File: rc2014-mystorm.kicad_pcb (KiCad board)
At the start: 2 copper layers, 100 x 50 mm, 25 parts, among them J1 FPGA connection, J2 Config, J3 Conn_01x05, J6 Extra, P1 RC2014 BUS, U1 SN74LVCC3245A, U2 SN74LVCC3245A, U3 SN74LVCC3245A, U4 SN74LVCC3245A, U5 SN74LVCC3245A, U6 LM1117-3.3

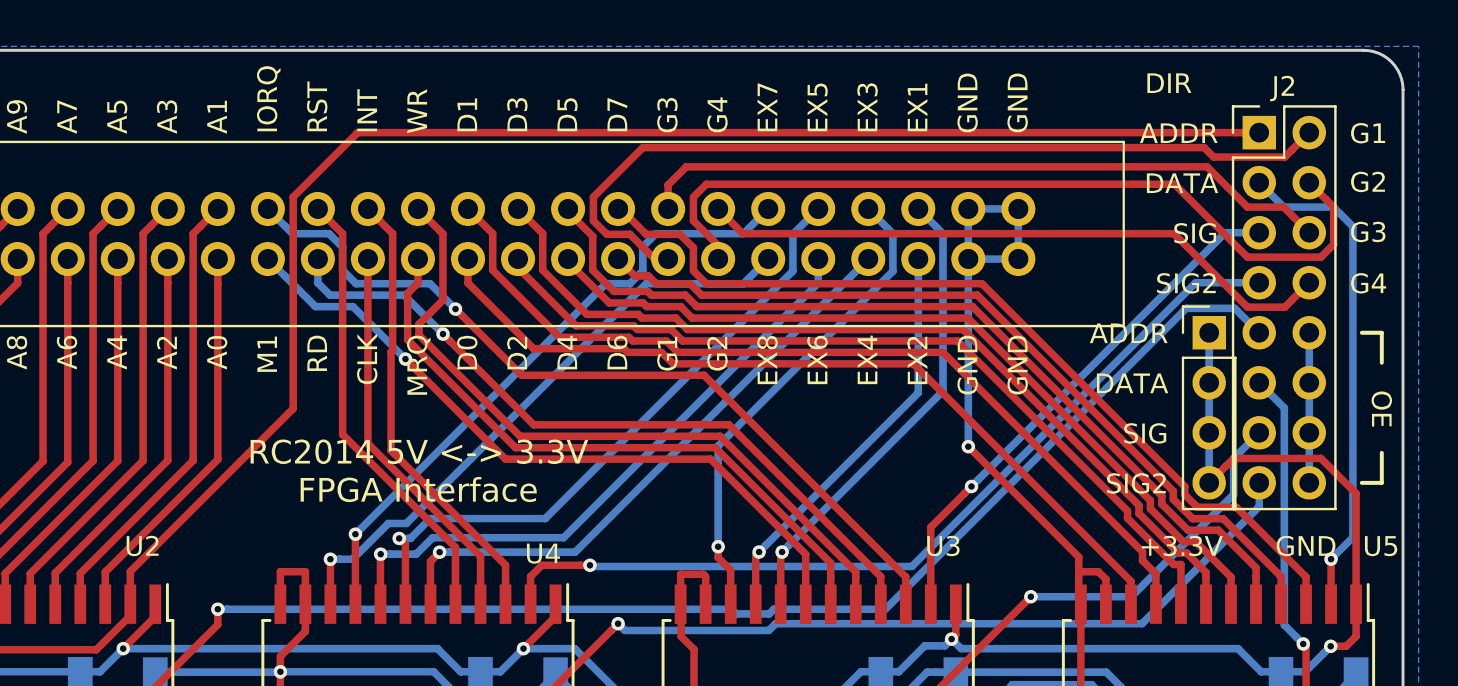
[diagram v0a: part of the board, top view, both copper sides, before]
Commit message: resave with kicad 9 and tidy up - no attempt made to update to new component libraries
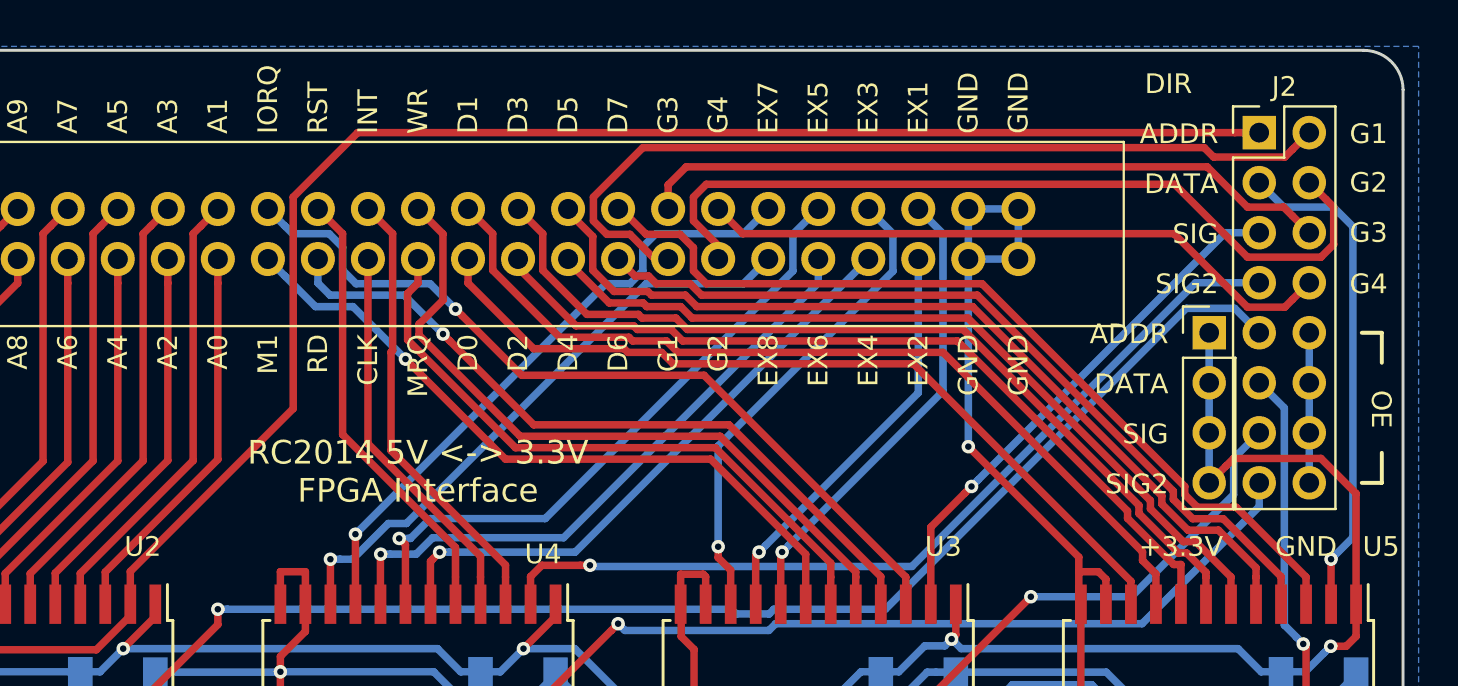
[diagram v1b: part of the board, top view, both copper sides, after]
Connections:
- net +3V3 renamed +3.3V
- net //IORQ renamed //IORQ
- net //IORQLV renamed //IORQLV
- net //RD renamed //RD
- net //RDLV renamed //RDLV
- net //RESET renamed //RESET
- net //RESETLV renamed //RESETLV
- net //WR renamed //WR
- net //WRLV renamed //WRLV
- P1 pad 37: Net-(P1-Pad37) -> unconnected-(P1-Pin_37-Pad37)
- P1 pad 38: Net-(P1-Pad38) -> unconnected-(P1-Pin_38-Pad38)
- P1 pad 39: Net-(P1-Pad39) -> unconnected-(P1-Pin_39-Pad39)
- U1 pad 23: Net-(U1-Pad23) -> unconnected-(U1-NC-Pad23)
- U2 pad 23: Net-(U2-Pad23) -> unconnected-(U2-NC-Pad23)
- U3 pad 23: Net-(U3-Pad23) -> unconnected-(U3-NC-Pad23)
- U4 pad 23: Net-(U4-Pad23) -> unconnected-(U4-NC-Pad23)
- U5 pad 23: Net-(U5-Pad23) -> unconnected-(U5-NC-Pad23)
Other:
- net class Default removed
- net class IO removed
- net class analogue removed
- net class gnd removed
- net class vcc removed
